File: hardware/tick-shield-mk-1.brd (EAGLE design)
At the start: 62 x 52 mm, 15 parts, among them IC1 DS1307, Y1 32.768kHz

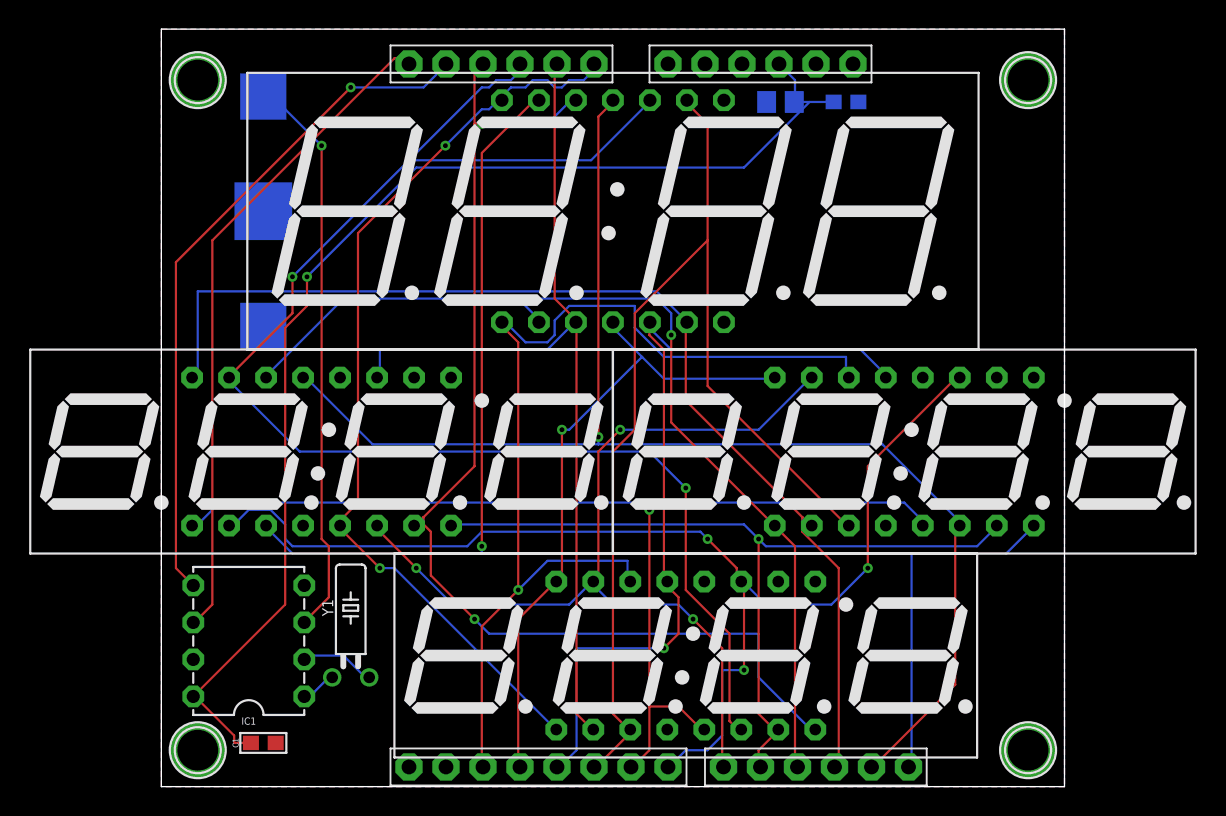
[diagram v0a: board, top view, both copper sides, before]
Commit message: shieldify all the things
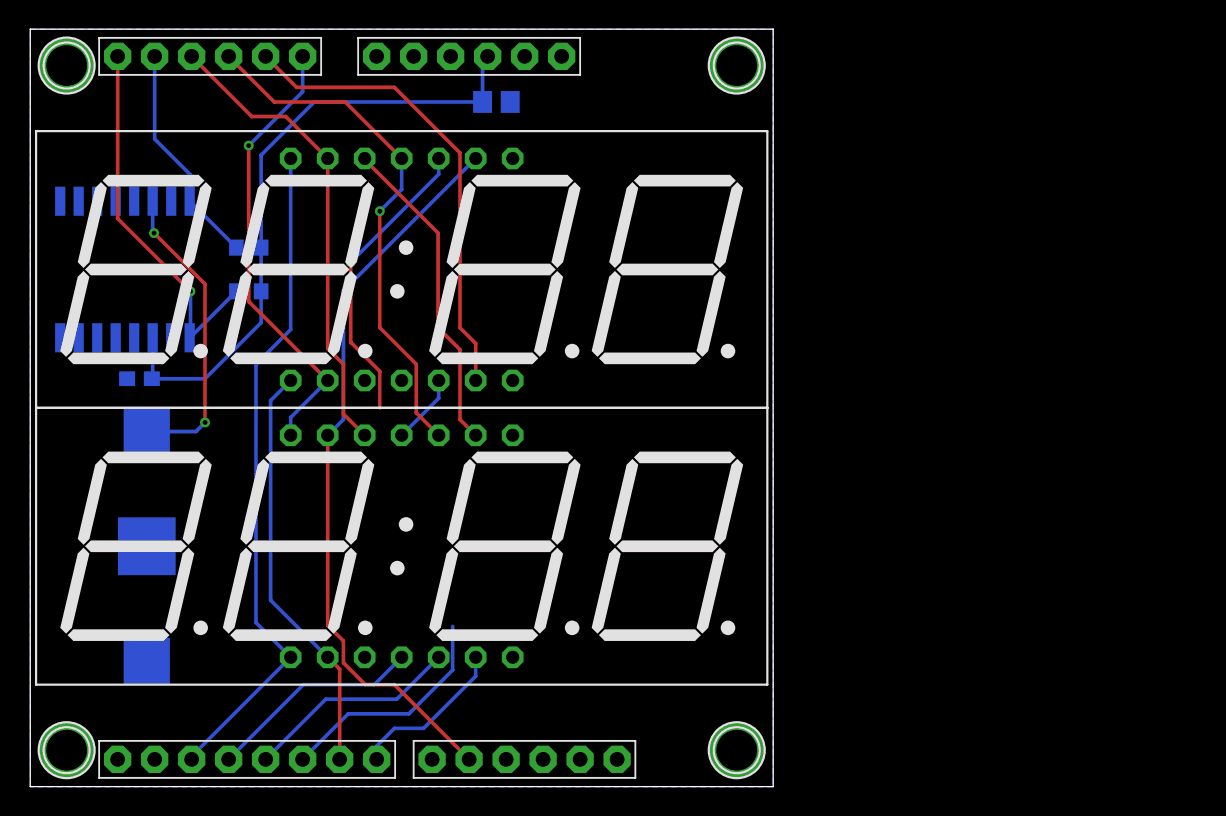
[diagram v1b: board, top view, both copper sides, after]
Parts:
- removed C3: 1uF, A_butts:C0805
- removed DISPLAY3, DISPLAY4: 7SEG_4DIGIT_COLON_APOS, A_butts:7SEG_4DIG_10MM
- removed Y1: 32.768kHz, A_butts:TC26H
- added R1, R2: 4.7k, A_butts:R0603
- C2: value 0.1uF -> 1uF; device A_butts:C0603 -> A_butts:C0805
- DISPLAY2: value 7SEG_4DIGIT_COLON_APOS -> 7SEG_4DIGIT_COLON14.2MM-CC; device A_butts:7SEG_4DIG_10MM -> A_butts:7SEG_4DIG_0.56IN_14MM_ADAFRUIT
- IC1: value DS1307 -> DS1338C; device A_butts:DIL08 -> A_butts:SO16W
- moved IC1 26.9 mm to (6.50, 35.5), flipped to the bottom, turned to 0 degrees
- moved C1 26.4 mm to (7.50, 28.0), flipped to the bottom
- moved BAT1 24.4 mm to (8.00, 16.5)
- moved C2 24.0 mm to (32.0, 47.0)
- moved H4 20.0 mm to (48.5, 49.5)
- moved SHIELD 20.0 mm to (6.00, 1.87)
- moved H3 20.0 mm to (48.5, 2.50)
- moved DISPLAY1 15.0 mm to (25.5, 35.5)
- moved H2 9.06 mm to (2.50, 49.5)
- moved H1 9.00 mm to (2.50, 2.50)
- moved DISPLAY2 8.51 mm to (25.5, 16.5)
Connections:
- removed net D10: DISPLAY1.P$13, DISPLAY2.14, DISPLAY3.1, SHIELD.D10
- removed net D11: DISPLAY1.P$9, DISPLAY2.16, DISPLAY3.2, SHIELD.D11
- removed net D12: DISPLAY1.P$4, DISPLAY2.13, DISPLAY3.6, SHIELD.D12
- removed net D13: DISPLAY1.P$2, DISPLAY2.3, DISPLAY3.8, SHIELD.D13
- removed net N$1: IC1.2, Y1.2
- removed net N$2: IC1.1, Y1.1
- net A0: now also DISPLAY1.P$13, DISPLAY2.P$1; no longer DISPLAY1.P$1, DISPLAY2.5, DISPLAY4.1
- net A1: now also DISPLAY1.P$9, DISPLAY2.P$12; no longer DISPLAY1.P$12, DISPLAY2.11, DISPLAY4.2
- net A2: now also DISPLAY1.P$4, DISPLAY2.P$5; no longer DISPLAY1.P$5, DISPLAY2.15, DISPLAY4.6
- net A3: now also DISPLAY1.P$2, DISPLAY2.P$3; no longer DISPLAY1.P$3, DISPLAY2.7, DISPLAY4.8
- net D2: now also DISPLAY1.P$1, DISPLAY2.P$14; no longer DISPLAY1.P$14, DISPLAY3.14, DISPLAY4.14
- net D3: now also DISPLAY1.P$12, DISPLAY2.P$11; no longer DISPLAY1.P$11, DISPLAY3.16, DISPLAY4.16
- net D4: now also DISPLAY1.P$5, DISPLAY2.P$10; no longer DISPLAY1.P$10, DISPLAY3.13, DISPLAY4.13
- net D5: now also DISPLAY1.P$3, DISPLAY2.P$6; no longer DISPLAY1.P$6, DISPLAY3.3, DISPLAY4.3
- net D6: now also DISPLAY1.P$14, DISPLAY2.P$13; no longer DISPLAY2.1, DISPLAY3.5, DISPLAY4.5
- net D7: now also DISPLAY1.P$11, DISPLAY2.P$9; no longer DISPLAY2.2, DISPLAY3.11, DISPLAY4.11
- net D8: now also DISPLAY1.P$10, DISPLAY2.P$4; no longer DISPLAY2.6, DISPLAY3.15, DISPLAY4.15
- net D9: now also DISPLAY1.P$6, DISPLAY2.P$2; no longer DISPLAY2.8, DISPLAY3.7, DISPLAY4.7
- net GND: now also IC1.10, IC1.11, IC1.12, IC1.13, IC1.15, IC1.5, IC1.6, IC1.7, IC1.8, IC1.9; no longer C3.2
- net N$3: now also IC1.14; no longer IC1.3
- net SCL: now also IC1.1, R2.1; no longer IC1.6
- net SDA: now also IC1.16, R1.1; no longer IC1.5
- net VCC: now also IC1.3, R1.2, R2.2; no longer C3.1, IC1.8
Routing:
- net D13: track 102.0 -> 0.00 mm, vias 1 -> 0
- net D12: track 92.8 -> 0.00 mm, vias 1 -> 0
- net D11: track 76.5 -> 0.00 mm
- net D7: track 82.3 -> 11.0 mm, vias 3 -> 0
- net D10: track 67.5 -> 0.00 mm, vias 1 -> 0
- net A2: track 102.4 -> 36.1 mm, vias 2 -> 1
- net D8: track 62.7 -> 4.81 mm, vias 3 -> 0
- net D6: track 75.0 -> 28.5 mm, vias 1 -> 0
- net A3: track 78.0 -> 32.3 mm, vias 2 -> 0
- net VCC: track 83.1 -> 43.4 mm, vias 1 -> 0
- net D5: track 74.4 -> 38.0 mm
- net A0: track 63.5 -> 30.8 mm, vias 2 -> 1
- net SDA: track 46.9 -> 15.5 mm, vias 1 -> 0
- net A1: track 63.2 -> 32.2 mm
- net D3: track 45.0 -> 14.8 mm, vias 1 -> 0
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- removed copper zone on layer 1, net GND
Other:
- board size 62 x 52 mm -> 51 x 52 mm
